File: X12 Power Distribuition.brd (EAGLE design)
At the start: 152.4 x 76.2 mm, 47 parts, among them Q1 SPB80P06P, Y1 ECS-80-S-4X

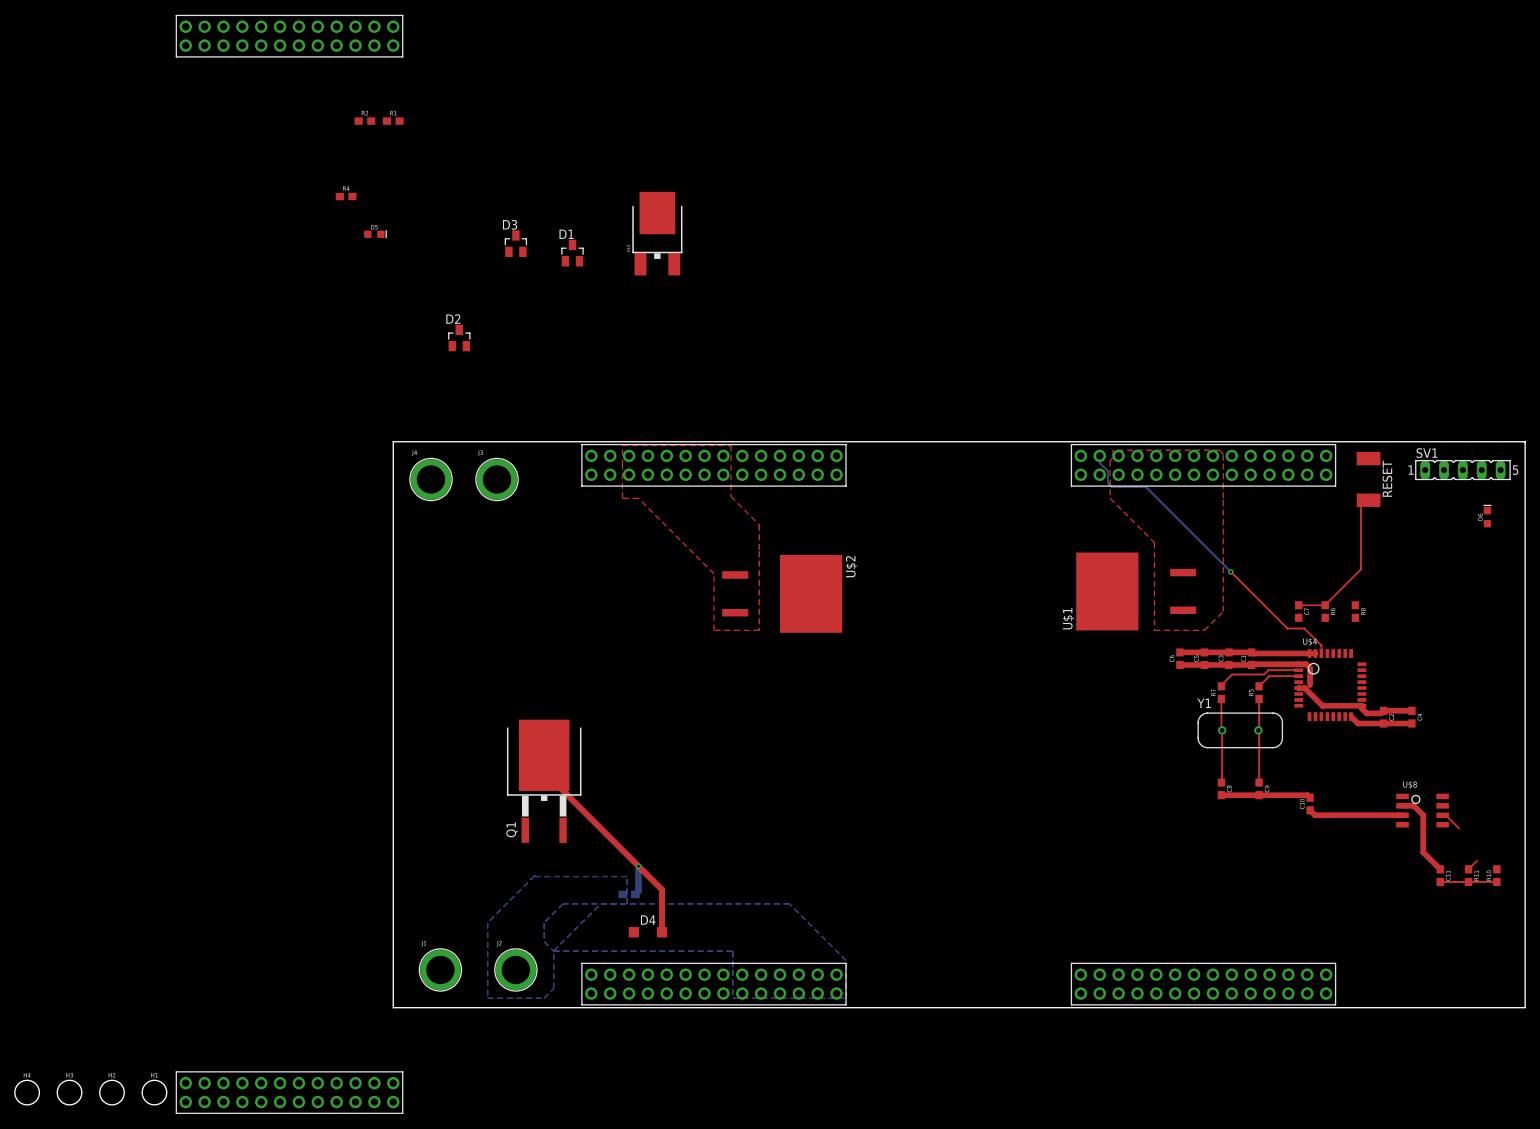
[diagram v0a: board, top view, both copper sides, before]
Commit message: Board
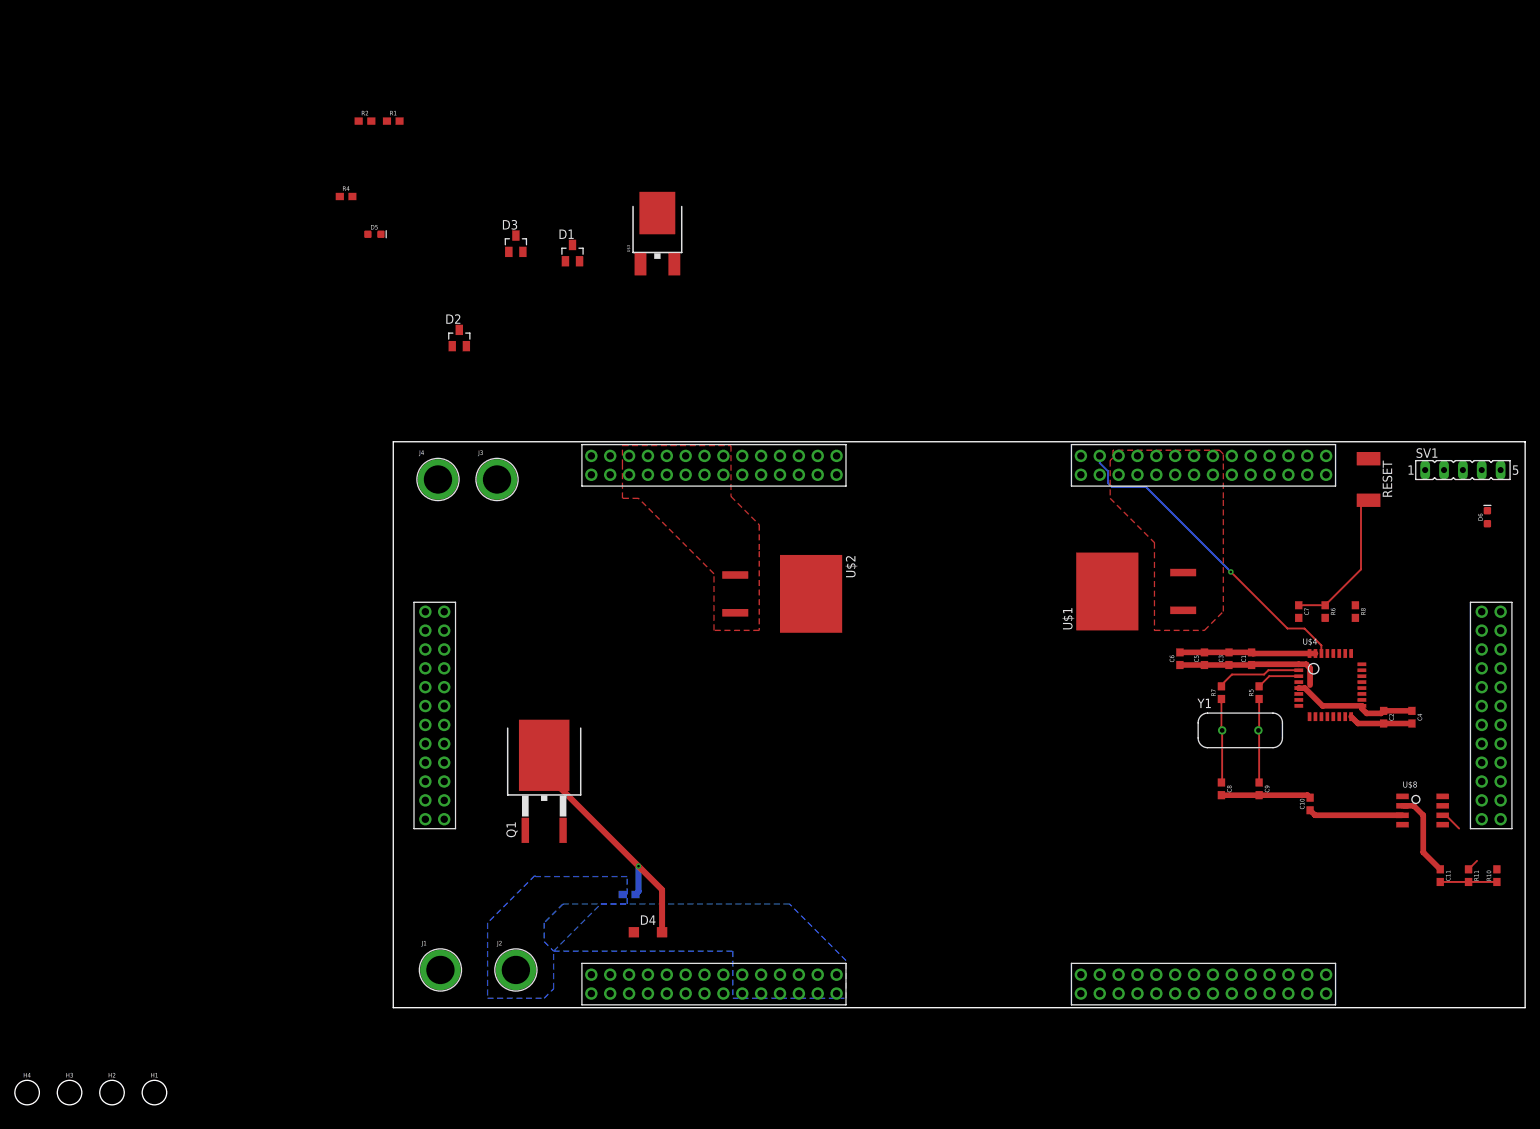
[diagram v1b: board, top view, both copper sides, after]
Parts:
- moved U$6 73.5 mm to (4.32, 53.3), turned to 270 degrees
- moved J4 0.94 mm to (6.02, 71.1)
